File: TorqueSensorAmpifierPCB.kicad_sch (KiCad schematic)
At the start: 17 parts, among them J1 Conn_01x04_Socket, J2 Conn_01x04_Socket, U1 LM386

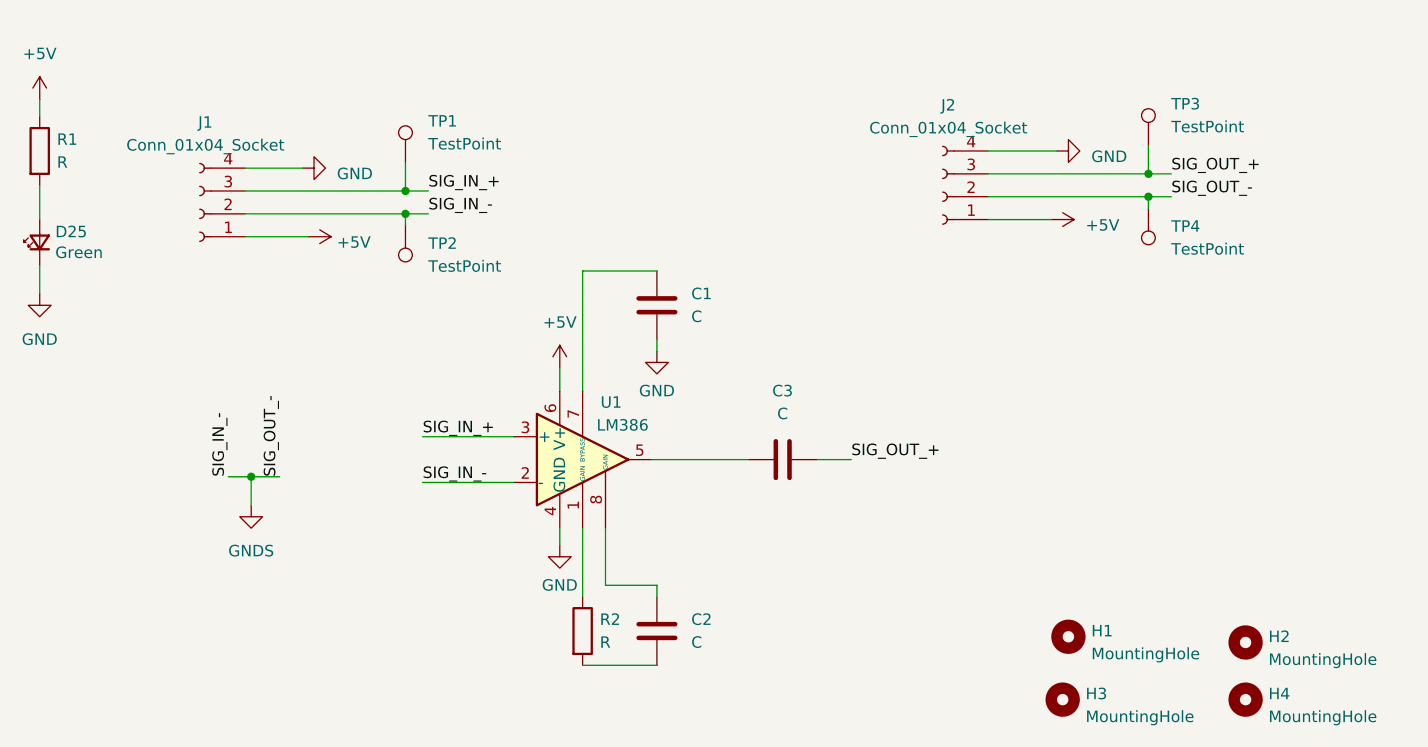
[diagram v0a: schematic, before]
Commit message: Added Gerbers
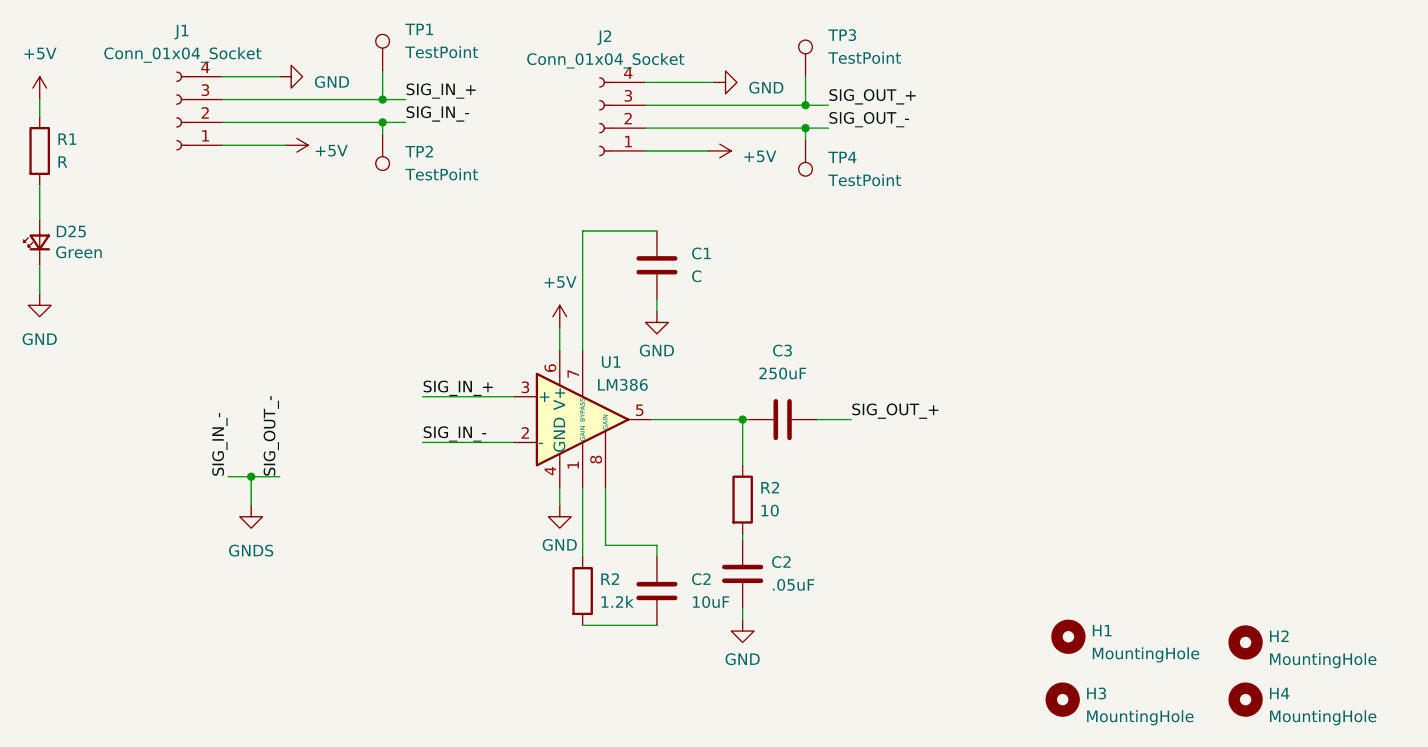
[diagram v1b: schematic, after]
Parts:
- added C2: .05uF, Capacitor_SMD:C_0805_2012Metric, symbol Device:C
- added R2: 10, Resistor_SMD:R_0805_2012Metric, symbol Device:R
- C2: value C -> 10uF
- C3: value C -> 250uF
- R1: footprint Resistor_SMD:R_0805_2012Metric -> Resistor_THT:R_Axial_DIN0614_L14.3mm_D5.7mm_P20.32mm_Horizontal
- R2: value R -> 1.2k
- U1: footprint Package_SO:SOIC-8-1EP_3.9x4.9mm_P1.27mm_EP2.41x3.3mm -> HCRL:M08A_TEX-L
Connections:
- net GND: now also C2.2
- net at C3.1, U1.5: now also R2.1
- new net: C2.1, R2.2
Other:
- moved on the sheet: C1, C2, C3, J1, J2, R2, TP1, TP2, TP3, TP4, U1
